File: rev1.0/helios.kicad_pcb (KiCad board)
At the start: 4 copper layers, 17.8 x 33 mm, 58 parts, among them J1 USB_C_Receptacle_USB2.0, J2 helios-pinout, Q1 2N7002VC-, Q2 2N7002VC-, SW1 SWITCH, U1 USBLC6-2P6, U2 LP5907SNX-3.3-NOPB, U3 W25Q128JVPIQ, U4 RP2040, U5 74LVC1T45, Y1 12MHz

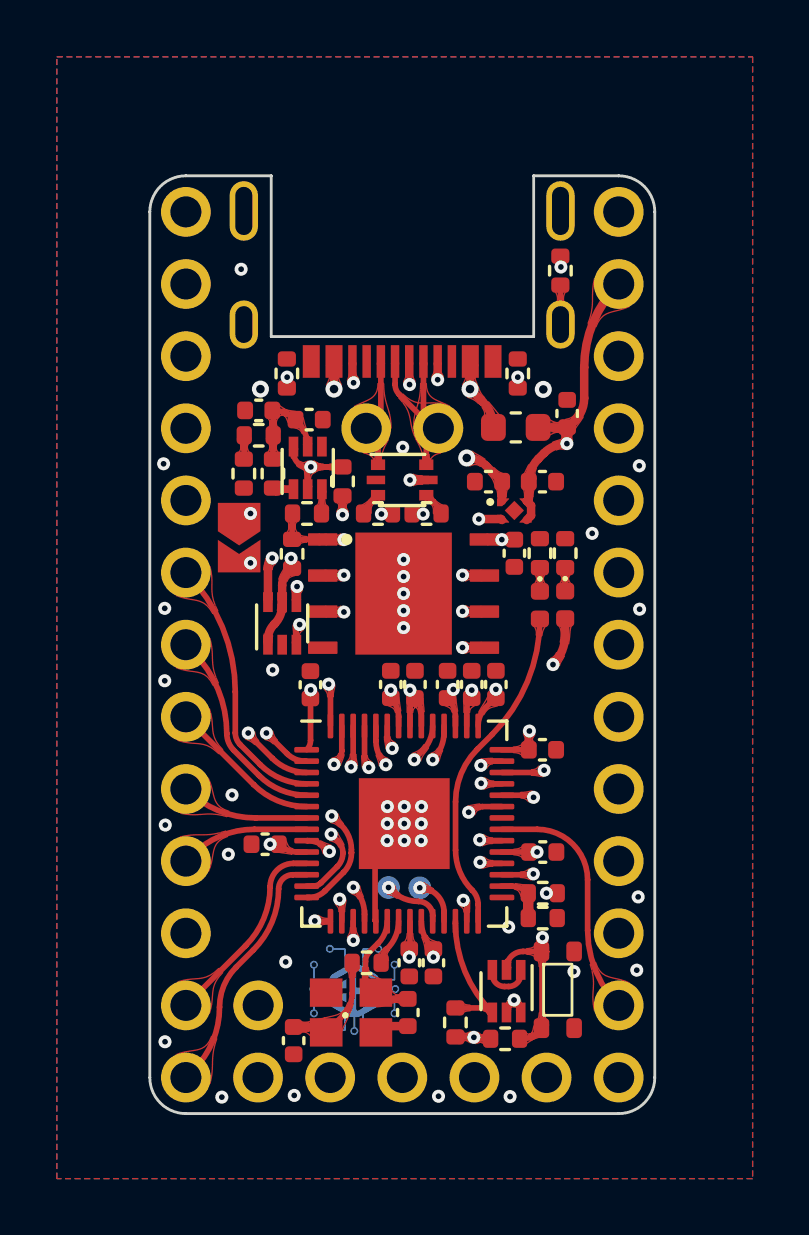
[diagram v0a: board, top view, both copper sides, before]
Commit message: added prod files for jlcpcb
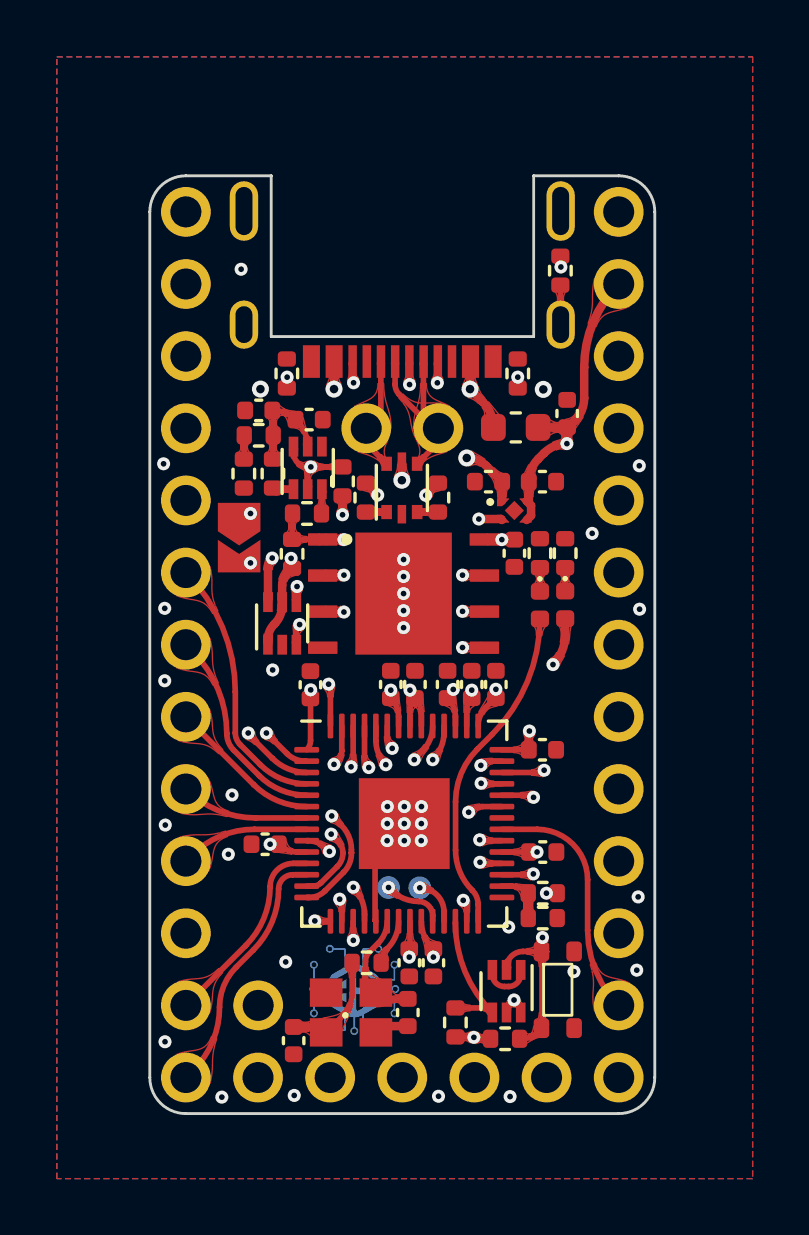
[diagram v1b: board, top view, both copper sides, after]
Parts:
- moved J1 4.75 mm to (158.9, 136.8)
- moved R12 0.71 mm to (157.6, 144.2), turned to 90 degrees
- moved R13 0.69 mm to (160.1, 144.2), turned to 90 degrees
- moved U1 0.28 mm to (158.8, 143.9), turned to 90 degrees
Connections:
- U1 pad 1: /PORT+ -> /USB+
- U1 pad 3: /USB+ -> /USB-
- U1 pad 4: /USB- -> /PORT-
- U1 pad 6: /PORT- -> /PORT+
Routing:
- net /D+: track 11.1 -> 12.0 mm
- net /D-: track 11.1 -> 12.0 mm
- net GND: vias 39 -> 38
